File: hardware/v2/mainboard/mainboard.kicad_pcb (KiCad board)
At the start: 2 copper layers, 17 parts, among them J1 LEG1_RJ11, J2 LEG2_RJ11, J3 LEG3_RJ11, J4 LEG4_RJ11, J5 LEG5_RJ11, J6 LEG6_RJ11, J7 SBEC_5V_IN, J9 IMU_I2C, U1 ESP32-WROOM-32D, U2 SP3485CN

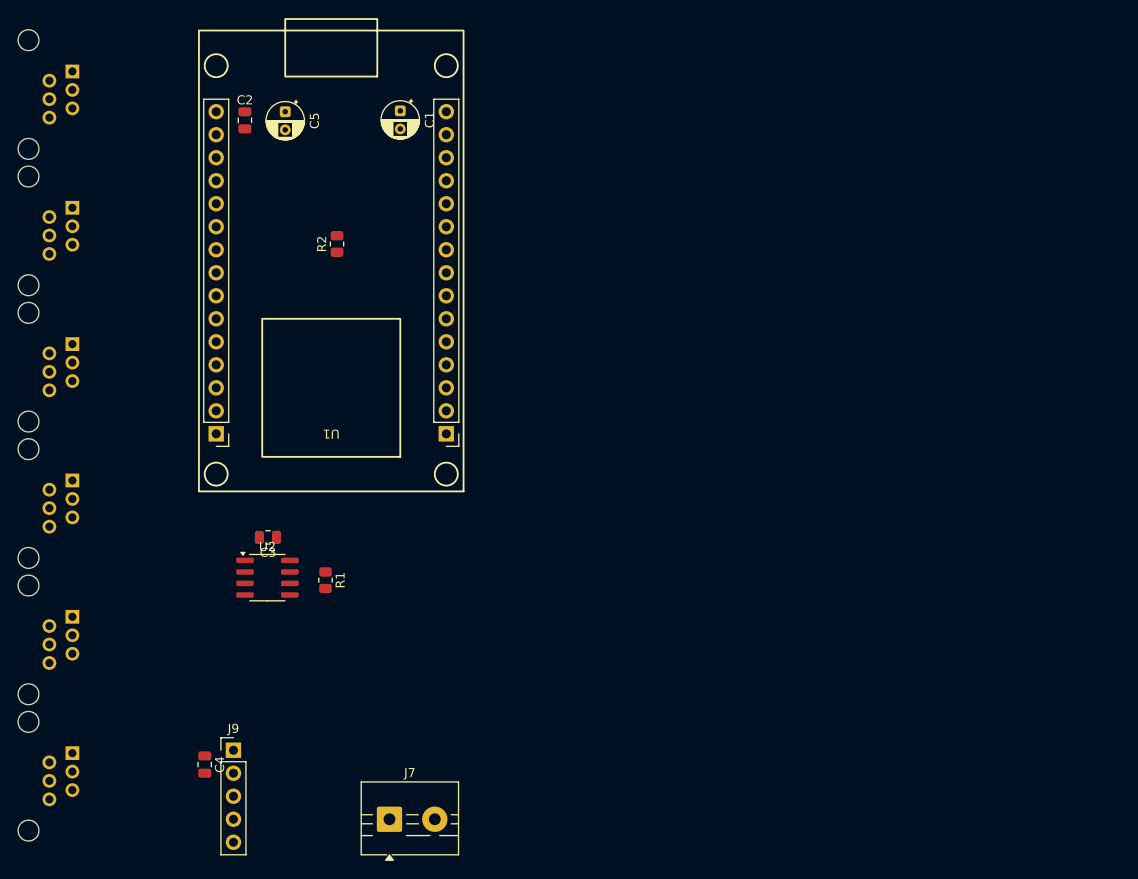
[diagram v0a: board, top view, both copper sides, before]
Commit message: mainboard physical design
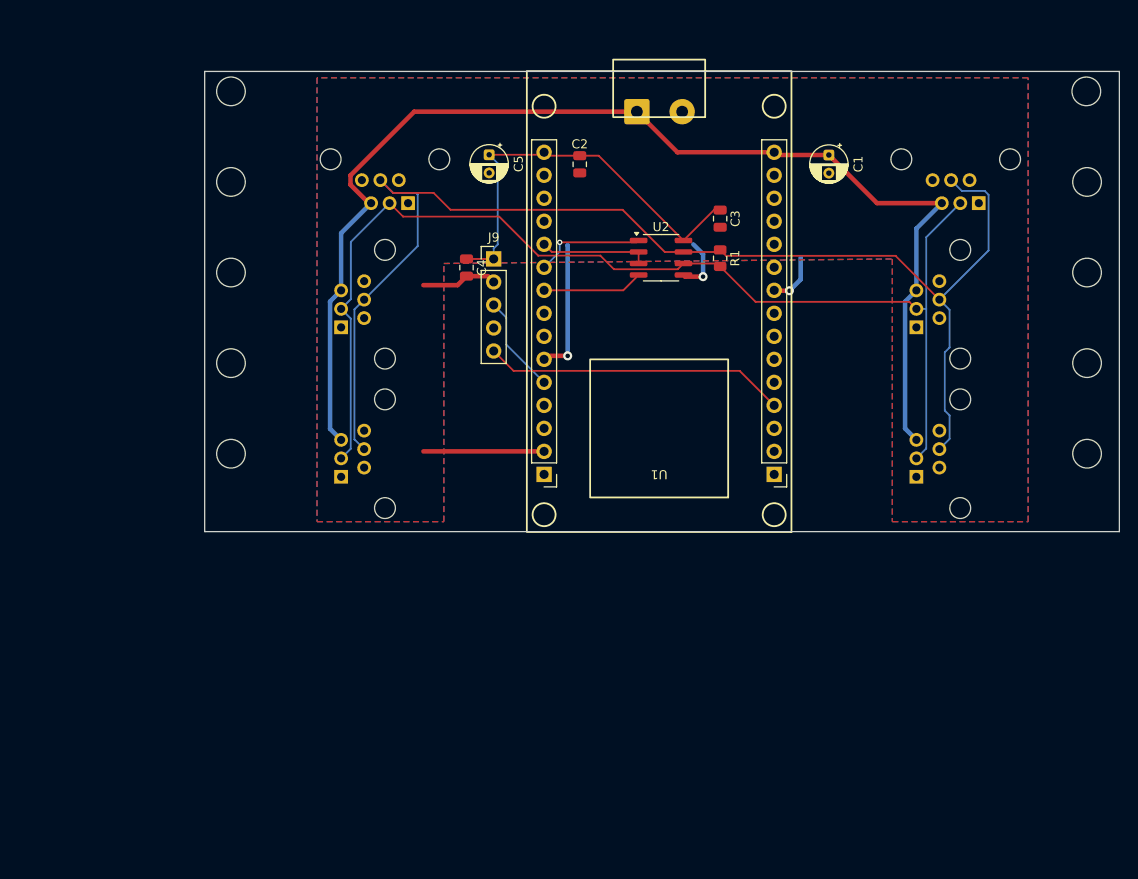
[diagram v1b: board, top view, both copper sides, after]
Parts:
- removed R2: 10k, Resistor_SMD:R_0805_2012Metric
- J7: moved to B.Cu
- moved J3 104.6 mm to (187.1, 65.3), turned to 0 degrees
- moved J2 98.5 mm to (180.2, 79.0), turned to -90 degrees
- moved J1 98.0 mm to (180.2, 95.5), turned to -90 degrees
- moved J7 82.7 mm to (149.3, 55.2)
- moved C4 62.0 mm to (130.5, 72.5)
- moved J9 61.4 mm to (133.5, 71.5)
- moved C3 61.1 mm to (158.5, 67.0), turned to -90 degrees
- moved R1 56.2 mm to (158.5, 71.4)
- moved U2 56.0 mm to (152.0, 71.4)
- moved J6 53.7 mm to (116.7, 95.5), turned to -90 degrees
- moved C1 47.6 mm to (170.5, 60.0)
- moved J4 40.2 mm to (124.0, 65.3), turned to 0 degrees
- moved C2 37.3 mm to (143.0, 61.0)
- moved U1 36.5 mm to (151.8, 95.3)
- moved J5 32.5 mm to (116.7, 79.0), turned to -90 degrees
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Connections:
- U1 pad 0: ESP_EN -> unconnected-(U1-EN-Pad0)
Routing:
- net RS485_B: track 0.00 -> 140.1 mm
- net +5V: track 0.00 -> 133.4 mm
- net RS485_A: track 0.00 -> 126.0 mm
- net GND: track 0.00 -> 48.9 mm, vias 0 -> 3
- net +3.3V: track 0.00 -> 46.1 mm
- net IMU_INT: track 0.00 -> 33.5 mm
- net ESP_RXD: track 0.00 -> 12.3 mm, vias 0 -> 1
- net RS485_DE: track 0.00 -> 12.1 mm
- net ESP_TXD: track 0.00 -> 11.1 mm
- net IMU_SDA: track 0.00 -> 10.8 mm
- added copper zone on B.Cu, net GND
- added copper zone on F.Cu, net GND
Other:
- board outline added: 101 x 50.8 mm
